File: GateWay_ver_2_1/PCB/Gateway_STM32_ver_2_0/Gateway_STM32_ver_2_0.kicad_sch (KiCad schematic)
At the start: 44 parts, among them J4 Conn_01x04, SW2 SW_Push, U7 STM32F407VETx, Y1 8mhz, Y2 Crystal_GND23

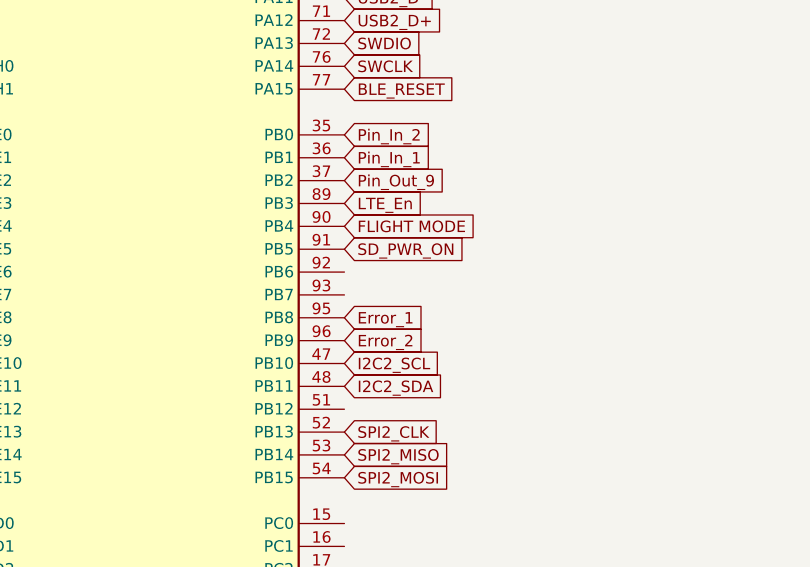
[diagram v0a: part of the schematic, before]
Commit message: 1
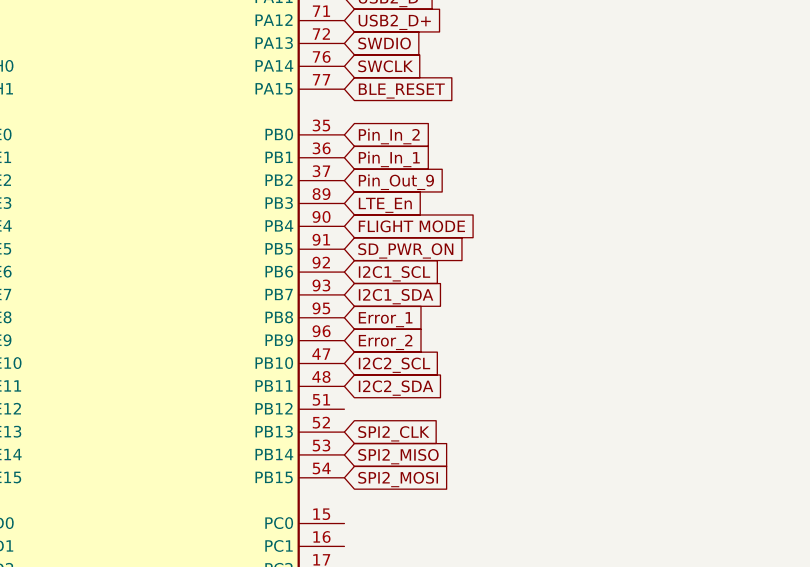
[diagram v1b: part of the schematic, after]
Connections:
- net I2C1_SCL: now reaches U7.92 (PB6)
- net I2C1_SDA: now reaches U7.93 (PB7)
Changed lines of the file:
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@@
     )
   )
+  (global_label "I2C1_SDA" (shape input) (at 114.046 112.268 0) (fields_autoplaced)
+    (effects (font (size 1.27 1.27)) (justify left))
+    (property "Intersheet References" "${INTERSHEET_REFS}" (id 0) (at 125.1997 112.3474 0)
+      (effects (font (size 1.27 1.27)) (justify left) hide)
+    )
+  )
   (global_label "LTE_RXD" (shape input) (at 68.326 152.908 180) (fields_autoplaced)
     (effects (font (size 1.27 1.27)) (justify right))
@@
     )
   )
+  (global_label "I2C1_SCL" (shape input) (at 114.046 109.728 0) (fields_autoplaced)
+    (effects (font (size 1.27 1.27)) (justify left))
+    (property "Intersheet References" "${INTERSHEET_REFS}" (id 0) (at 125.1392 109.8074 0)
+      (effects (font (size 1.27 1.27)) (justify left) hide)
+    )
+  )
   (global_label "UART_MLTPX_1_RX" (shape input) (at 68.326 160.528 180) (fields_autoplaced)
     (effects (font (size 1.27 1.27)) (justify right))
@@
       (reference "#PWR0313") (unit 1) (value "+3.3V") (footprint "")
     )
-    (path "/8944a068-f989-4394-a0e4-fb891ac82c67/d60193f4-8481-4abd-b144-cbba3dc6e1a6"
-      (reference "#PWR0314") (unit 1) (value "GND") (footprint "")
-    )
-    (path "/8944a068-f989-4394-a0e4-fb891ac82c67/03268d63-11ef-442a-9ae1-385f65e666f1"
-      (reference "#PWR0315") (unit 1) (value "GND") (footprint "")
-    )
-    (path "/8944a068-f989-4394-a0e4-fb891ac82c67/8fc16aad-3e04-42af-a4dd-d9579404b0ad"
-      (reference "#PWR0316") (unit 1) (value "+3.3V") (footprint "")
-    )
-    (path "/8944a068-f989-4394-a0e4-fb891ac82c67/79c80a96-370f-415e-8dc3-d5c70f9f4e93"
-      (reference "#PWR0317") (unit 1) (value "GND") (footprint "")
-    )
     (path "/17dbbc3f-e526-4f0c-aeef-1a51fbd344a5/44e527b0-0c19-4642-86b3-bad529530e43"
       (reference "#PWR0319") (unit 1) (value "+5V") (footprint "")
@@
       (reference "#PWR0378") (unit 1) (value "GND") (footprint "")
     )
+    (path "/8944a068-f989-4394-a0e4-fb891ac82c67/171d3809-7193-4a1d-97d9-b497e023538c"
+      (reference "#PWR?") (unit 1) (value "+3.3V") (footprint "")
+    )
+    (path "/8944a068-f989-4394-a0e4-fb891ac82c67/673b2a00-38e5-42e2-b3a2-cb225a9dac0c"
+      (reference "#PWR?") (unit 1) (value "GND") (footprint "")
+    )
+    (path "/8944a068-f989-4394-a0e4-fb891ac82c67/c24562ae-1a7d-4fd2-a19d-e9310c020e51"
+      (reference "#PWR?") (unit 1) (value "+3.3V") (footprint "")
+    )
+    (path "/8944a068-f989-4394-a0e4-fb891ac82c67/e36955a8-0ed3-4fa3-8419-5c604980f71d"
+      (reference "#PWR?") (unit 1) (value "+3.3V") (footprint "")
+    )
     (path "/019ca31f-c666-4ad4-9da0-821bbd7be497/6ad2d142-1fc3-46bf-a53a-85bb7855cba5"
       (reference "AE1") (unit 1) (value "Antenna_Shield") (footprint "Connector_Coaxial:SMA_Amphenol_901-144_Vertical")
@@
       (reference "R107") (unit 1) (value "10k") (footprint "Resistor_SMD:R_0603_1608Metric")
     )
+    (path "/8944a068-f989-4394-a0e4-fb891ac82c67/89b7ef7a-1e1e-4928-8844-e031057845ce"
+      (reference "R?") (unit 1) (value "4.7k") (footprint "Resistor_SMD:R_0603_1608Metric")
+    )
+    (path "/8944a068-f989-4394-a0e4-fb891ac82c67/c622c683-d198-4cf8-8a64-19b64b6c1454"
+      (reference "R?") (unit 1) (value "4.7k") (footprint "Resistor_SMD:R_0603_1608Metric")
+    )
     (path "/dd619e6a-a0e1-4beb-8356-bcf75161c392/577f4706-5d40-4538-9616-d5b6ad5ea9f6"
       (reference "SW1") (unit 1) (value "SW_Push") (footprint "Button_Switch_SMD:SW_SPST_CK_RS282G05A3")
@@
       (reference "U25") (unit 1) (value "RT9742AGJ5F") (footprint "Package_TO_SOT_SMD:TSOT-23-5")
     )
-    (path "/8944a068-f989-4394-a0e4-fb891ac82c67/742aa22e-6c07-4a50-85eb-9780989225b7"
-      (reference "U26") (unit 1) (value "24AA02E48") (footprint "Package_TO_SOT_SMD:SOT-23-6")
+    (path "/8944a068-f989-4394-a0e4-fb891ac82c67/b39ba55e-e622-450c-aca4-8aea53a36aee"
+      (reference "U?") (unit 1) (value "24AA02E48") (footprint "Package_TO_SOT_SMD:SOT-23-5")
     )
     (path "/8832c854-dd5b-4a42-8207-a65f82d7dd7a"
